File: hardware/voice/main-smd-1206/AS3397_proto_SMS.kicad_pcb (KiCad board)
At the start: 2 copper layers, 71.1 x 104.1 mm, 105 parts, among them J1 ES, Q1 BS170F, Q2 BS170F, Q3 BS170F, Q4 BS170F, Q5 BS170F, U1 MCP6002, U2 Pico, U3 MCP6002, U4 MCP6002, U5 MCP6002, U6 74HC4050, U7 MCP6002

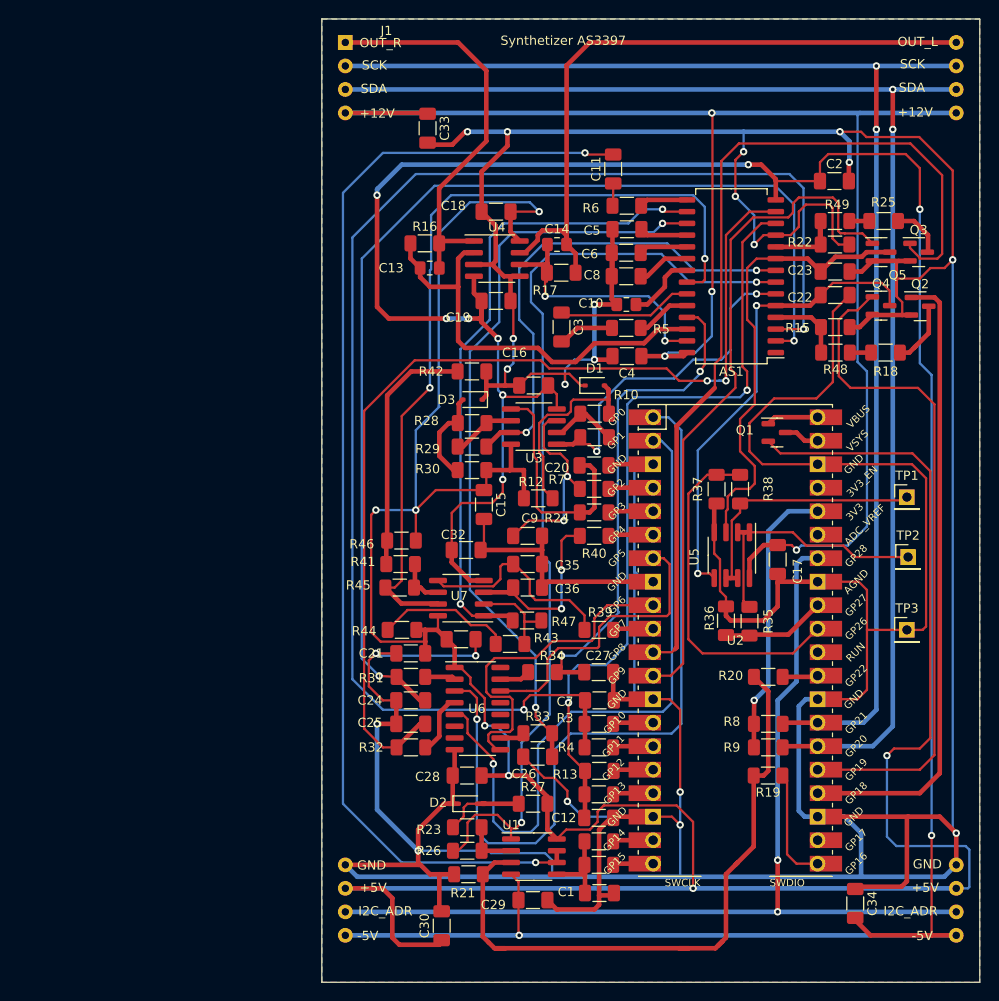
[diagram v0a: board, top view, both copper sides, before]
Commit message: Modif of voice board smd and Cleanup
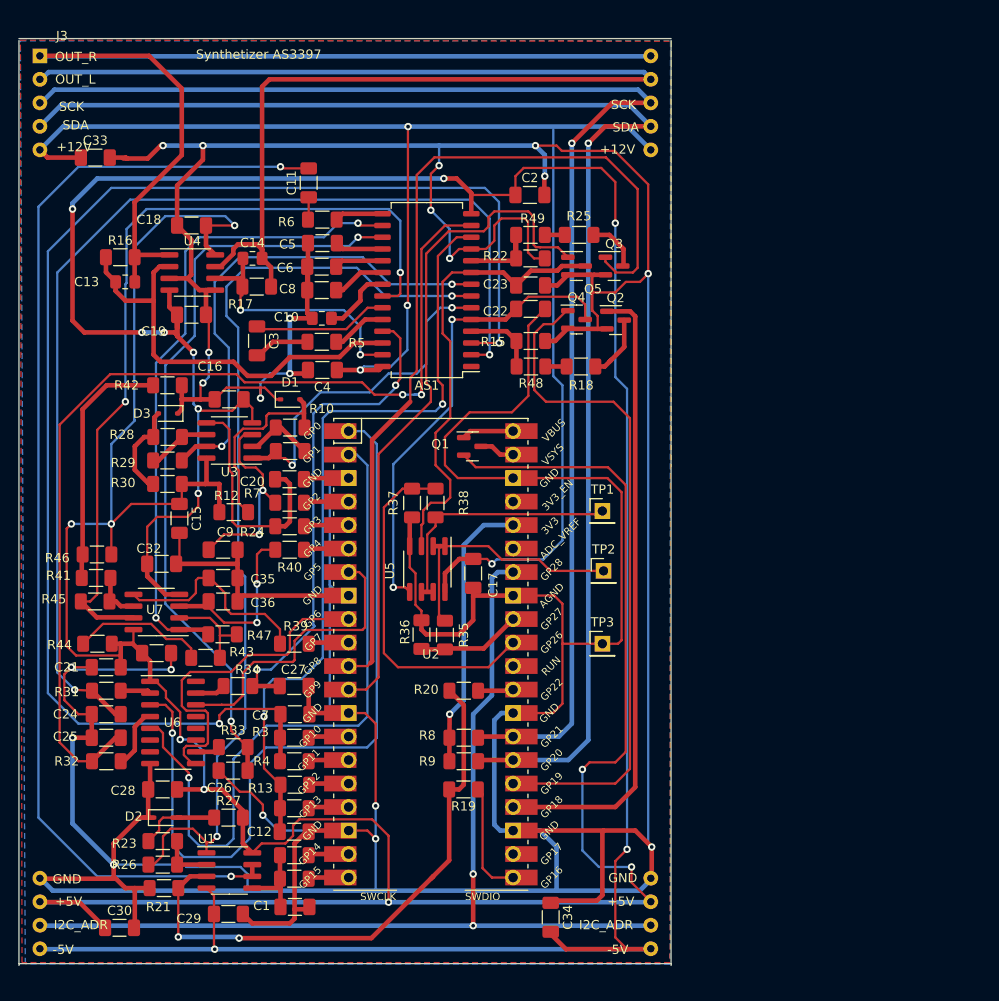
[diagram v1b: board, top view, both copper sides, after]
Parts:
- removed J1: ES, SYNTHFILLE:DIP-16_AS
- added J3: Conn_02x09_Counter_Clockwise, AS3397_proto_SMS:DIP-18_AS, F.Cu at (48.3, 47.2)
- R16, R17: value 100k -> 50k
- U1, U3, U5, U7: value MCP6002 -> TS922
- U4: value MCP6002 -> TL072
- moved C33 36.1 mm to (54.3, 58.2), turned to 0 degrees
- moved C30 34.8 mm to (56.9, 141.4), turned to 0 degrees
- moved AS1 33.0 mm to (90.1, 72.5)
- moved C1 33.0 mm to (75.8, 139.2)
- moved C10 33.0 mm to (78.7, 75.5)
- moved C11 33.0 mm to (77.3, 60.9)
- moved C12 33.0 mm to (75.8, 131.0)
- moved C13 33.0 mm to (57.5, 71.6)
- moved C14 33.0 mm to (71.2, 69.1)
- moved C15 33.0 mm to (63.3, 97.2)
- moved C18 33.0 mm to (64.7, 65.5)
- moved C19 33.0 mm to (64.7, 75.2)
- moved C26 33.0 mm to (69.2, 124.4)
- moved C27 33.0 mm to (75.8, 115.3)
- moved C35 33.0 mm to (68.1, 103.6)
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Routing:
- net OUT_R: track 43.8 -> 109.7 mm
- net OUT_L: track 73.5 -> 138.7 mm
- net Net-(U1A-+): track 100.5 -> 63.7 mm, vias 0 -> 2
- net +5V: track 322.3 -> 310.5 mm, vias 7 -> 8
- net I2C_SDA: track 147.7 -> 152.8 mm, vias 2 -> 1
- net I2C_SCK: track 146.4 -> 151.1 mm, vias 2 -> 1
- net +12V: track 172.2 -> 169.6 mm
- net GND: track 748.8 -> 750.6 mm
- net -5V: track 312.1 -> 313.2 mm
- added copper zone on F.Cu, net GND
- removed copper zone on F.Cu, net (none)
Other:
- board size 71.1 x 104.1 mm -> 70.5 x 100.2 mm
